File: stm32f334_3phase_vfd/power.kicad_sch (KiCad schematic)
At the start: 4 parts, among them U201 STGIB15CH60TS-L, U202 CC6903SO-x0A, U203 CC6903SO-x0A, U204 CC6903SO-x0A

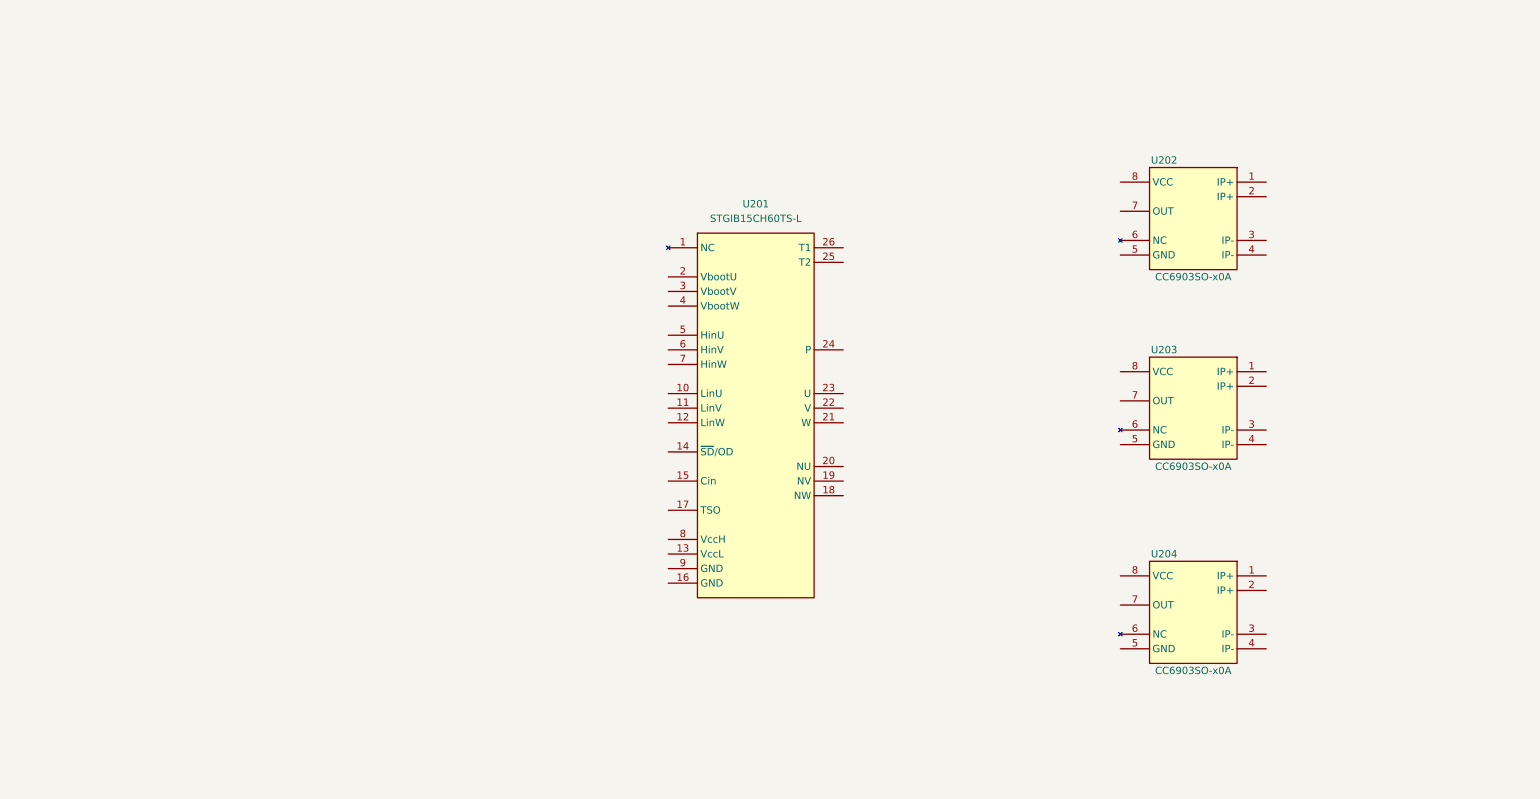
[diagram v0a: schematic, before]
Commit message: continue schematic work
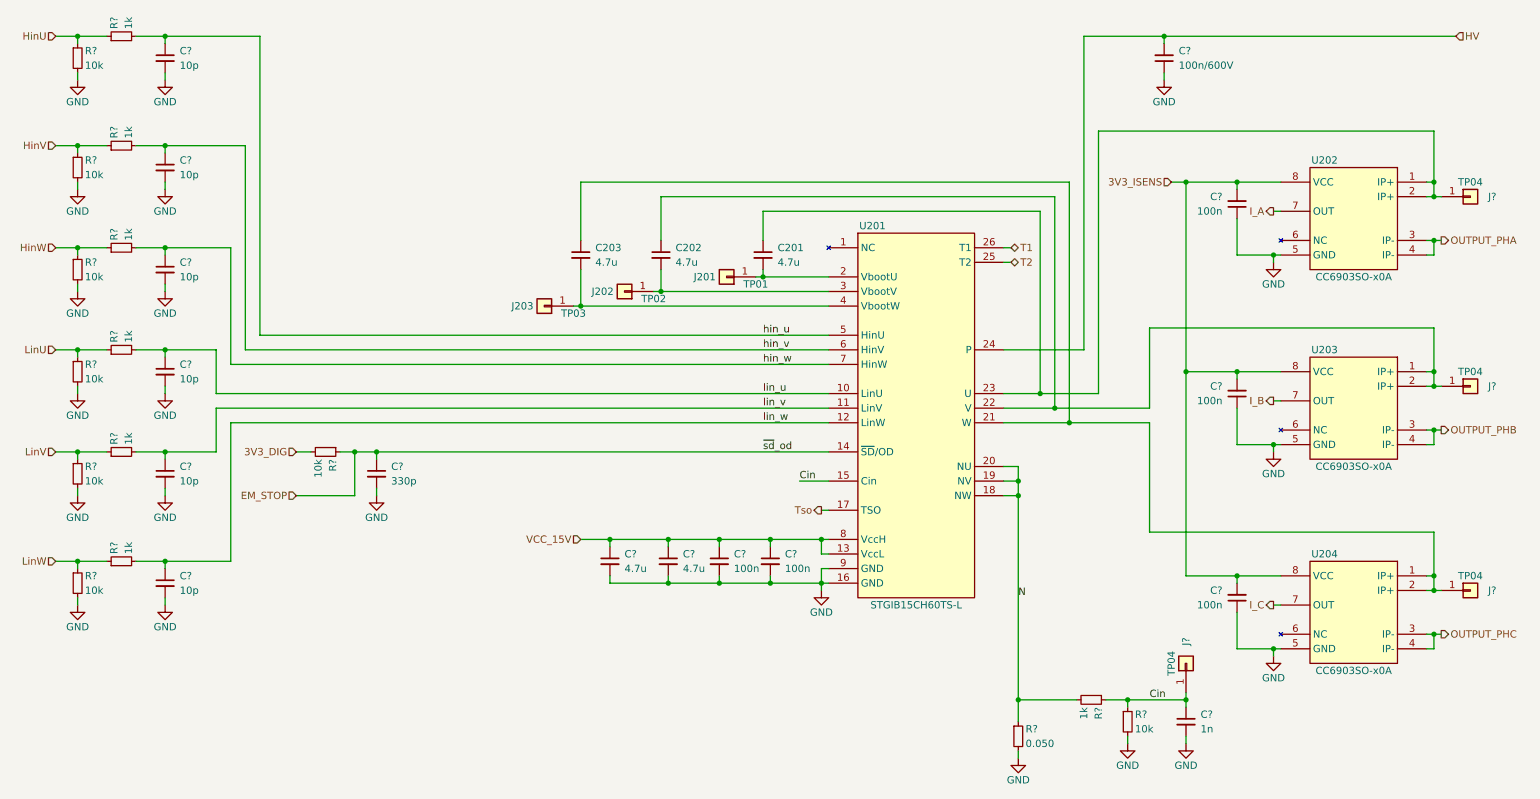
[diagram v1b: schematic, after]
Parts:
- added C201, C202, C203: 4.7u, symbol Device:C_Small
- added C? (x6): 10p, Capacitor_SMD:C_1206_3216Metric, symbol Device:C_Small
- added C? (x2): 4.7u, Capacitor_SMD:C_1206_3216Metric, symbol Device:C_Small
- added C? (x5): 100n, Capacitor_SMD:C_1206_3216Metric, symbol Device:C_Small
- added C?: 330p, Capacitor_SMD:C_1206_3216Metric, symbol Device:C_Small
- added C?: 1n, Capacitor_SMD:C_1206_3216Metric, symbol Device:C_Small
- added C?: 100n/600V, Capacitor_SMD:C_1206_3216Metric, symbol Device:C_Small
- added J201: TP01, symbol Connector_Generic:Conn_01x01
- added J202: TP02, symbol Connector_Generic:Conn_01x01
- added J203: TP03, symbol Connector_Generic:Conn_01x01
- added J? (x4): TP04, symbol Connector_Generic:Conn_01x01
- added R?: 0.050, symbol Device:R_Small
- added R? (x2): 10k, symbol Device:R_Small
- added R? (x6): 1k, Resistor_SMD:R_1206_3216Metric, symbol Device:R_Small
- added R? (x6): 10k, Resistor_SMD:R_1206_3216Metric, symbol Device:R_Small
- added R?: 1k, symbol Device:R_Small
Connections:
- net at U203.1 (IP+): now also U201.22 (V), U203.2 (IP+), C202.1, J?.1 (Pin_1)
- net OUTPUT_PHB: now reaches U203.3 (IP-)
- net OUTPUT_PHB: now also U203.4 (IP-)
- net GND: now reaches U203.5 (GND)
- net GND: now also U201.16 (GND), U201.9 (GND), U202.5 (GND), U204.5 (GND), C?.1, C?.1, C?.1, C?.1, C?.2, C?.2, C?.2, C?.2, C?.2, C?.2, C?.2, C?.2, C?.2, C?.2, C?.2, C?.2, R?.2, R?.2, R?.2, R?.2, R?.2, R?.2, R?.2, R?.2
- net I_B: now reaches U203.7 (OUT)
- net 3V3_ISENS: now reaches U203.8 (VCC)
- net 3V3_ISENS: now also U202.8 (VCC), U204.8 (VCC), C?.2, C?.2, C?.2
- net lin_u: now reaches U201.10 (LinU)
- net lin_u: now also C?.1, R?.2
- net lin_v: now reaches U201.11 (LinV)
- net lin_v: now also C?.1, R?.2
- net lin_w: now reaches U201.12 (LinW)
- net lin_w: now also C?.1, R?.2
- net VCC_15V: now reaches U201.13 (VccL)
- net VCC_15V: now also U201.8 (VccH), C?.1, C?.1, C?.1, C?.1
- net EM_STOP: now reaches U201.14 (~{SD}/OD)
- net EM_STOP: now also C?.1, R?.1
- net Cin: now reaches U201.15 (Cin)
- net Cin: now also C?.1, J?.1 (Pin_1), R?.1, R?.1
- net Tso: now reaches U201.17 (TSO)
- net N: now reaches U201.18 (NW)
- net N: now also U201.19 (NV), U201.20 (NU), R?.1, R?.2
- net at U201.2 (VbootU): now also C201.2, J201.1 (Pin_1)
- net at U201.21 (W): now also U204.1 (IP+), U204.2 (IP+), C203.1, J?.1 (Pin_1)
- net at U201.23 (U): now also U202.1 (IP+), U202.2 (IP+), C201.1, J?.1 (Pin_1)
- net HV: now reaches U201.24 (P)
- net HV: now also C?.2
- net T2: now reaches U201.25 (T2)
- net T1: now reaches U201.26 (T1)
- net at U201.3 (VbootV): now also C202.2, J202.1 (Pin_1)
- net at U201.4 (VbootW): now also C203.2, J203.1 (Pin_1)
- net hin_u: now reaches U201.5 (HinU)
- net hin_u: now also C?.1, R?.2
- net hin_v: now reaches U201.6 (HinV)
- net hin_v: now also C?.1, R?.2
- net hin_w: now reaches U201.7 (HinW)
- net hin_w: now also C?.1, R?.2
- net OUTPUT_PHC: now reaches U204.3 (IP-)
- net OUTPUT_PHC: now also U204.4 (IP-)
- net I_C: now reaches U204.7 (OUT)
- net OUTPUT_PHA: now reaches U202.3 (IP-)
- net OUTPUT_PHA: now also U202.4 (IP-)
- net I_A: now reaches U202.7 (OUT)
- new net 3V3_DIG: R?.2
- new net HinU: R?.1, R?.1
- new net HinV: R?.1, R?.1
- new net HinW: R?.1, R?.1
- new net LinU: R?.1, R?.1
- new net LinV: R?.1, R?.1
- new net LinW: R?.1, R?.1
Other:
- moved on the sheet: U201, U202, U203, U204
